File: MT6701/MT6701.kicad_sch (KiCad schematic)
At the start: 5 parts, among them J1 Conn_01x04_Socket, Q1 AS5048B-HTSP-500

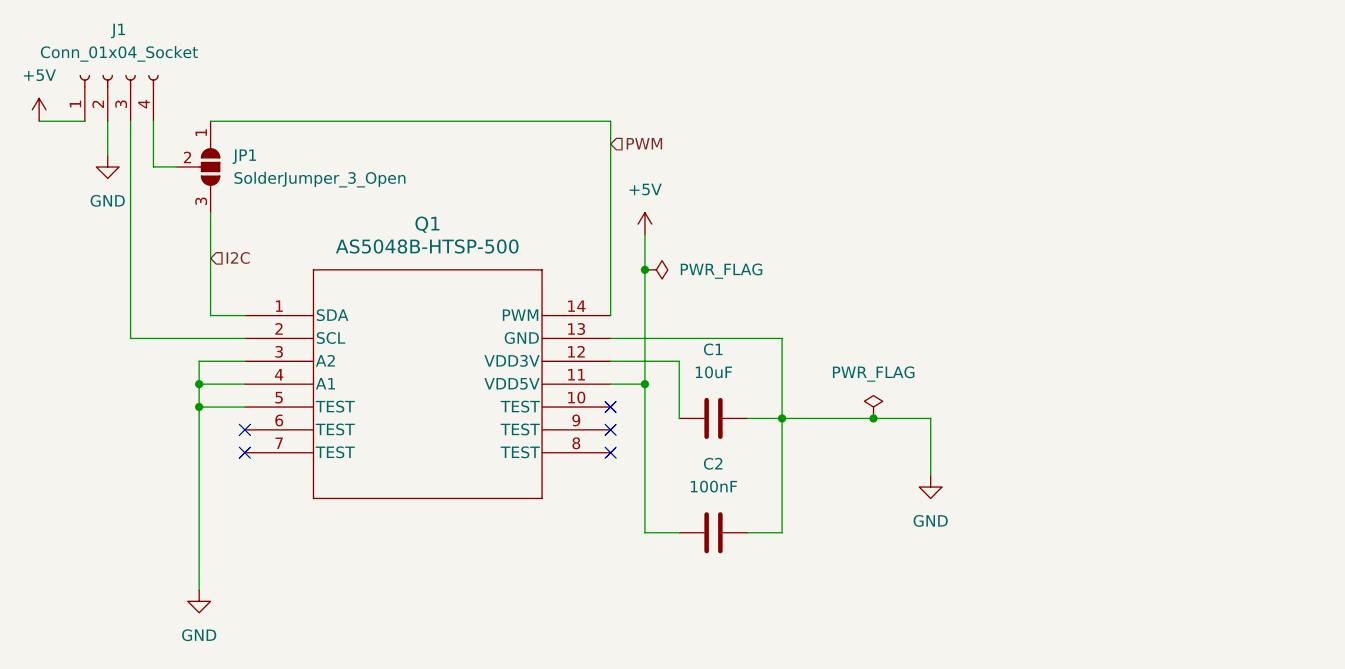
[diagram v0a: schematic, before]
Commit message: Updated Schematic
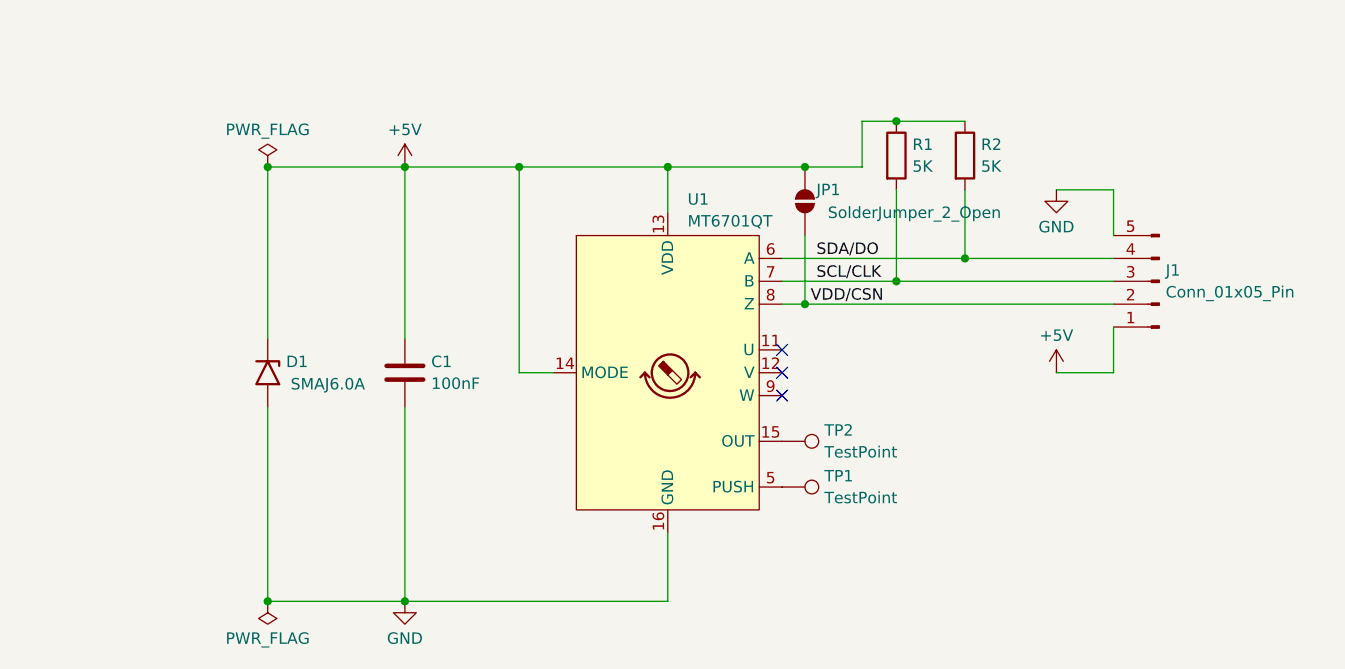
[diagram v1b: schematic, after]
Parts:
- removed C2: 100nF, Capacitor_SMD:C_0603_1608Metric, symbol Device:C
- removed J1: Conn_01x04_Socket, Connector_JST:JST_GH_SM04B-GHS-TB_1x04-1MP_P1.25mm_Horizontal, symbol Connector:Conn_01x04_Socket
- removed JP1: SolderJumper_3_Open, Jumper:SolderJumper-3_P1.3mm_Open_RoundedPad1.0x1.5mm, symbol Jumper:SolderJumper_3_Open
- removed Q1: AS5048B-HTSP-500, TRANS_HTSP-500_AMS, symbol Ethan:AS5048B-HTSP-500
- added D1: SMAJ6.0A, Diode_SMD:D_SMA, symbol Diode:SMAJ6.0A
- added J1: Conn_01x05_Pin, Connector_JST:JST_GH_SM05B-GHS-TB_1x05-1MP_P1.25mm_Horizontal, symbol Connector:Conn_01x05_Pin
- added JP1: SolderJumper_2_Open, symbol Jumper:SolderJumper_2_Open
- added R1, R2: 5K, symbol Device:R
- added TP1, TP2: TestPoint, symbol Connector:TestPoint
- added U1: MT6701QT, Package_DFN_QFN:QFN-16-1EP_3x3mm_P0.5mm_EP1.7x1.7mm, symbol Sensor_Magnetic:MT6701QT
- C1: value 10uF -> 100nF; footprint Capacitor_SMD:C_0603_1608Metric -> (none); Comment 10uF, X5R 6.3V -> (none); LCSC Part Number C95839 -> (none)
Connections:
- net +5V: now also C1.1, D1.1 (A1), J1.1 (Pin_1), JP1.2 (B), R1.1, R2.1, U1.13 (VDD), U1.14 (MODE)
- net GND: now also C1.2, D1.2 (A2), J1.5 (Pin_5), U1.16 (GND), U1.17 (GND); no longer C1.1
- new net: TP2.1, U1.15 (OUT)
- new net: TP1.1, U1.5 (PUSH)
- new net SCL/CLK: J1.3 (Pin_3), R1.2, U1.7 (B)
- new net SDA/DO: J1.4 (Pin_4), R2.2, U1.6 (A)
- new net VDD/CSN: J1.2 (Pin_2), JP1.1 (A), U1.8 (Z)
- no-connect marks 5 -> 3
